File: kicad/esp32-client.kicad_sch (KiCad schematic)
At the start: 1 part, among them U1 ESP32-C3-MINI-1

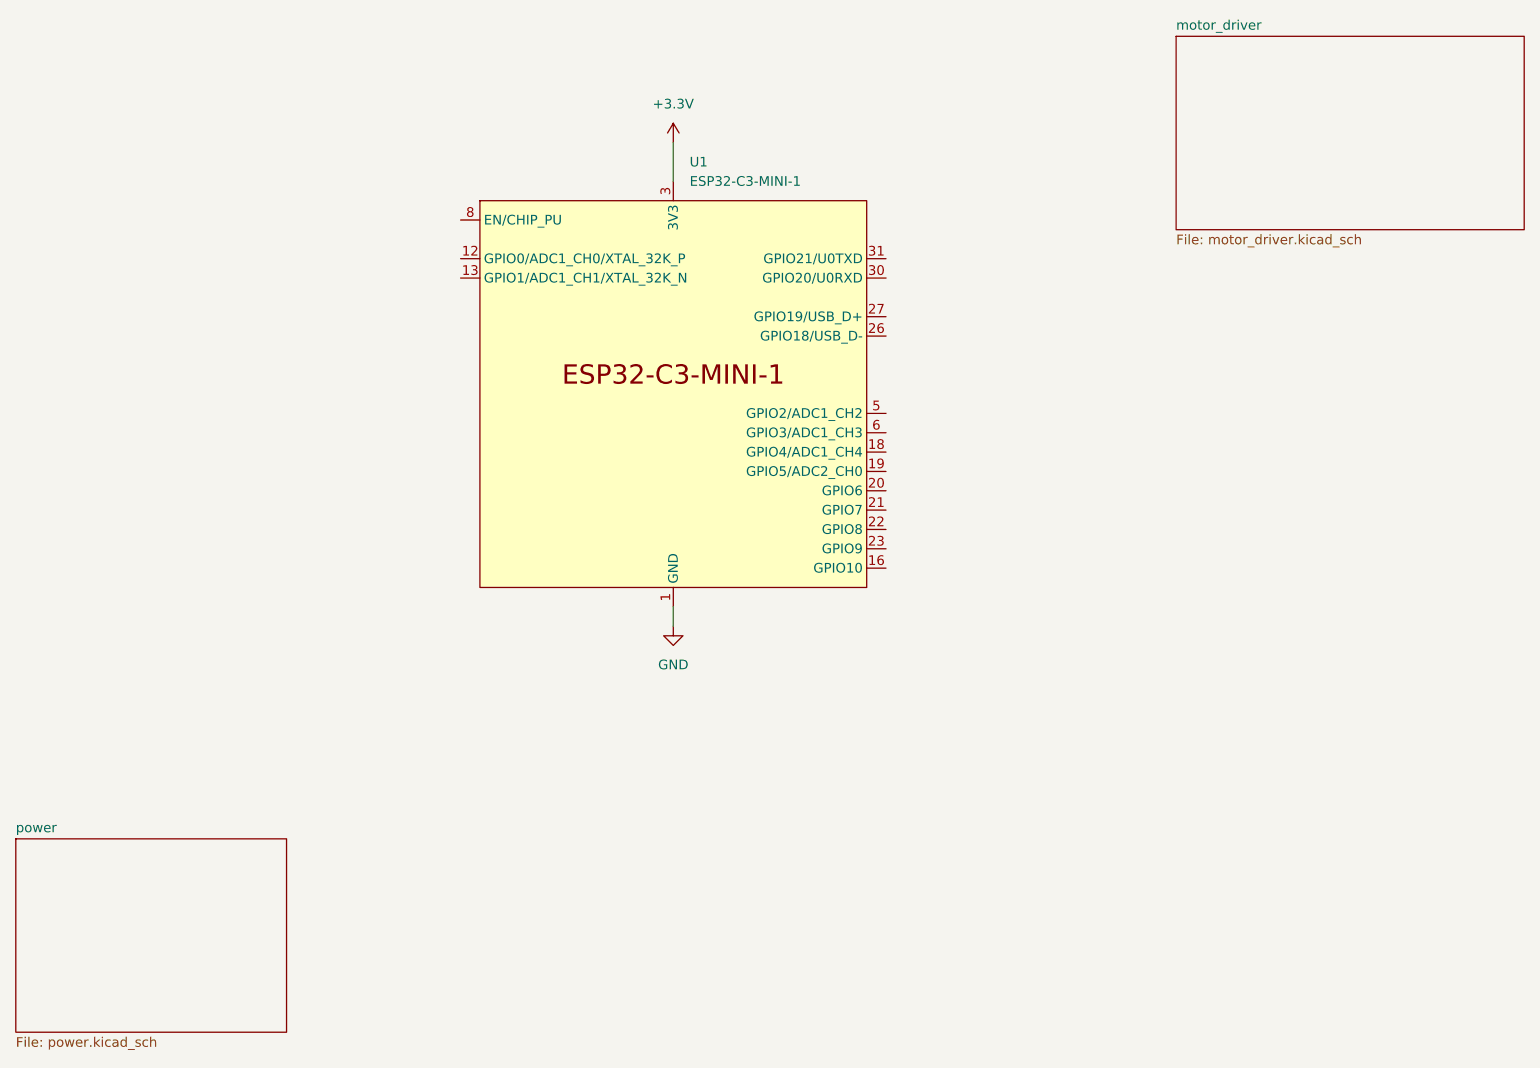
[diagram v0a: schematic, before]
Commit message: init
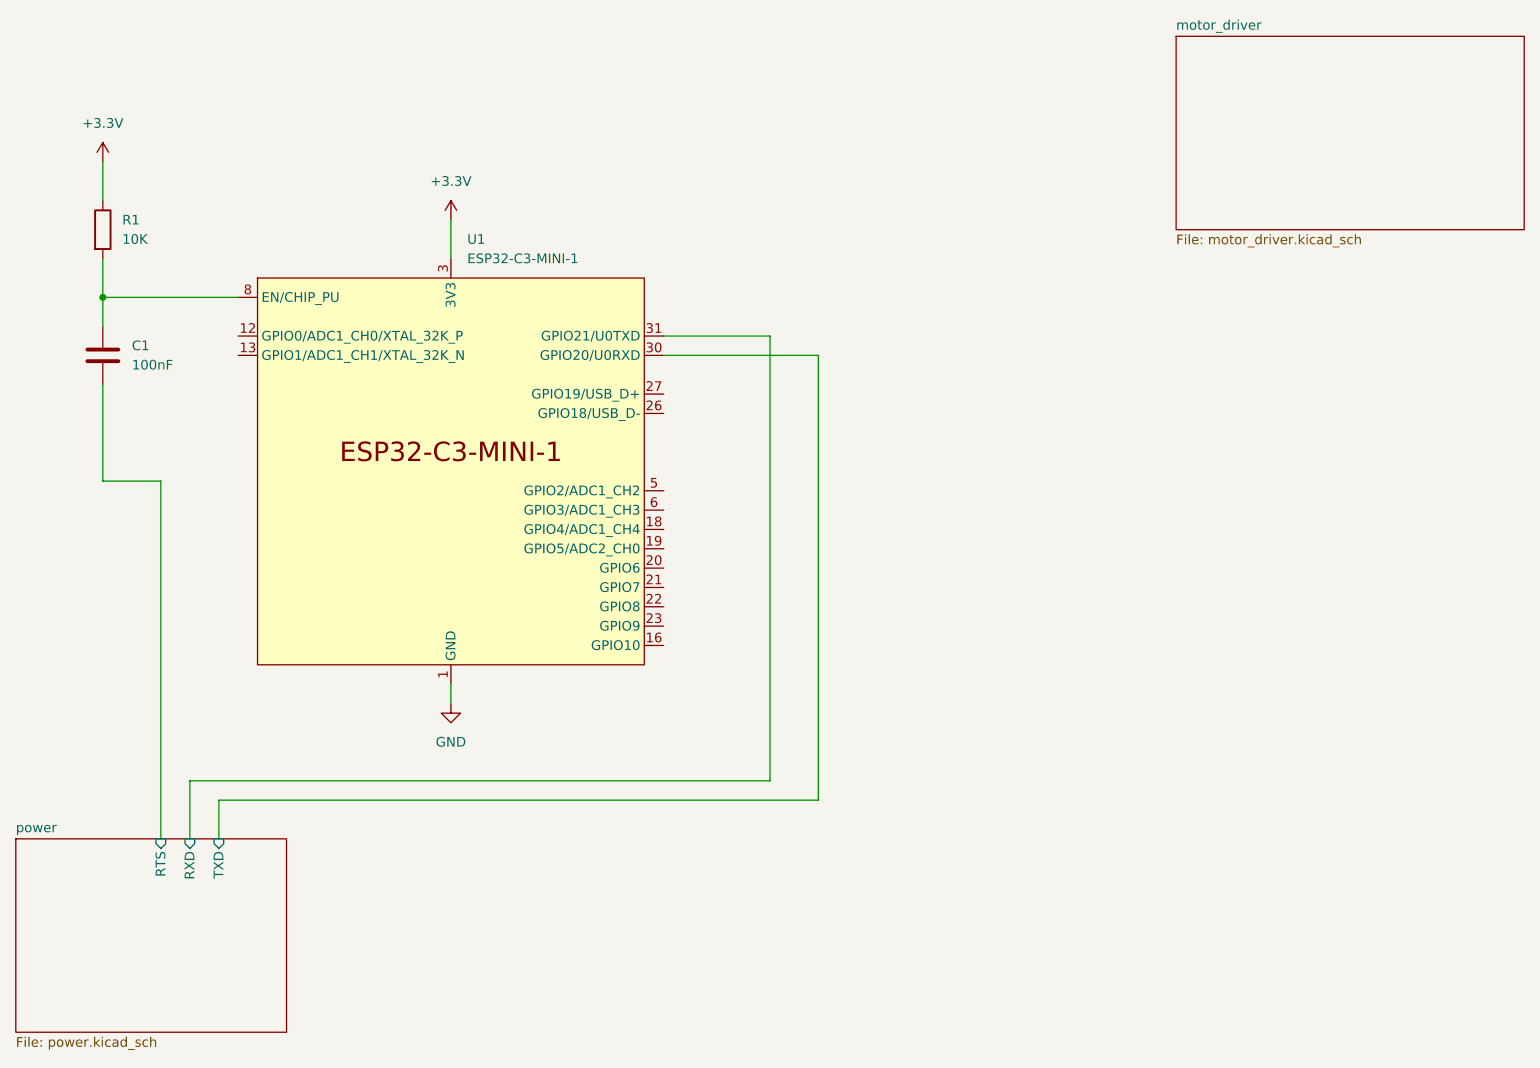
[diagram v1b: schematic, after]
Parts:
- added C1: 100nF, symbol Device:C
- added R1: 10K, symbol Device:R
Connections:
- net +3.3V: now also R1.1
- net power/TXD: now reaches U1.30 (GPIO20/U0RXD)
- net power/RXD: now reaches U1.31 (GPIO21/U0TXD)
- net at U1.8 (EN/CHIP_PU): now also C1.1, R1.2
- new net power/RTS: C1.2
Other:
- sheet power ports: added RTS, RXD, TXD; removed none
- moved on the sheet: U1

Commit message: init
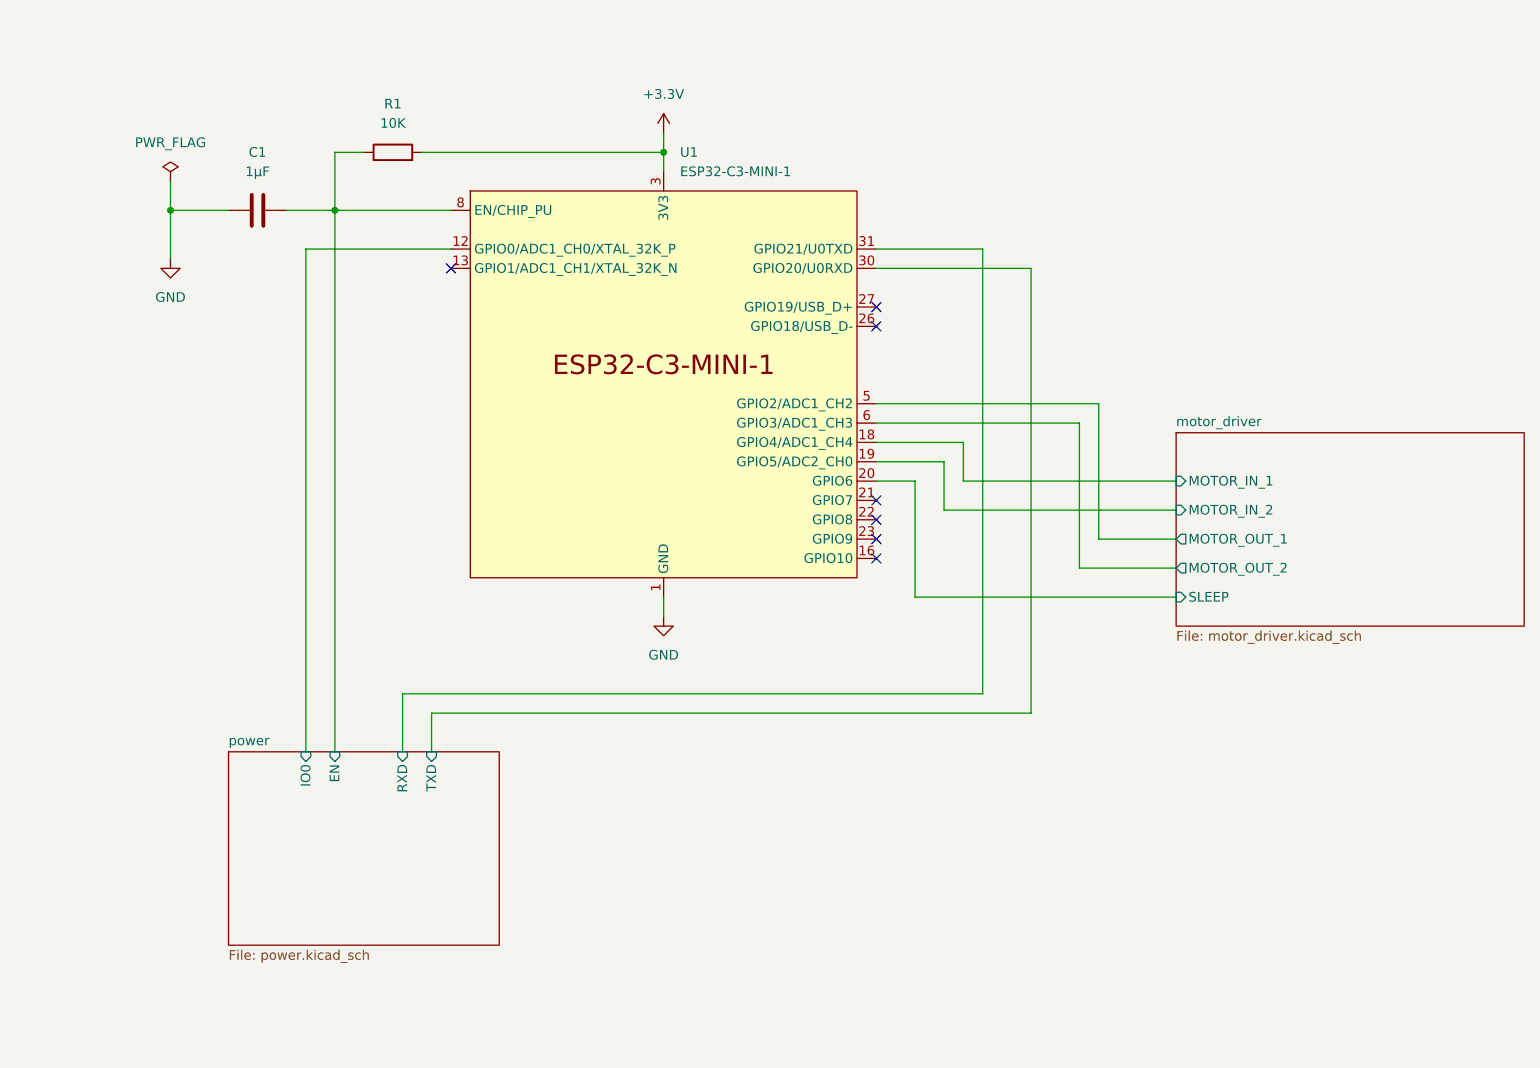
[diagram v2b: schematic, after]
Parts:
- C1: value 100nF -> 1µF; footprint (none) -> Capacitor_SMD:C_1206_3216Metric
- R1: footprint (none) -> Resistor_SMD:R_0805_2012Metric
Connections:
- net power/RTS is gone; now on net GND: C1.2
- net +3.3V: now also R1.2; no longer R1.1
- net power/EN: now reaches C1.1, U1.8 (EN/CHIP_PU)
- net power/EN: now also R1.1; no longer R1.2
- net power/IO0: now reaches U1.12 (GPIO0/ADC1_CH0/XTAL_32K_P)
- net motor_driver/MOTOR_IN_1: now reaches U1.18 (GPIO4/ADC1_CH4)
- net motor_driver/MOTOR_IN_2: now reaches U1.19 (GPIO5/ADC2_CH0)
- net motor_driver/SLEEP: now reaches U1.20 (GPIO6)
- net motor_driver/MOTOR_OUT_1: now reaches U1.5 (GPIO2/ADC1_CH2)
- net motor_driver/MOTOR_OUT_2: now reaches U1.6 (GPIO3/ADC1_CH3)
- no-connect marks 0 -> 7
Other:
- sheet motor_driver ports: added MOTOR_IN_1, MOTOR_IN_2, MOTOR_OUT_1, MOTOR_OUT_2, SLEEP; removed none
- sheet power ports: added EN, IO0; removed RTS
- moved on the sheet: U1
